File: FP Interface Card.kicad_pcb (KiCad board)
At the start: 6 copper layers, 90.2 x 101.1 mm, 40 parts, among them J100 ZX62-AB-5PA(31), P1 Card Edge for HSEC8-160-01-S-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, Q100 BC847BM3T5G, Q101 BC847BM3T5G, Q102 BC847BM3T5G, Q103 BC847BM3T5G, SW100 SW_Push_SPST, U100 AP2161W

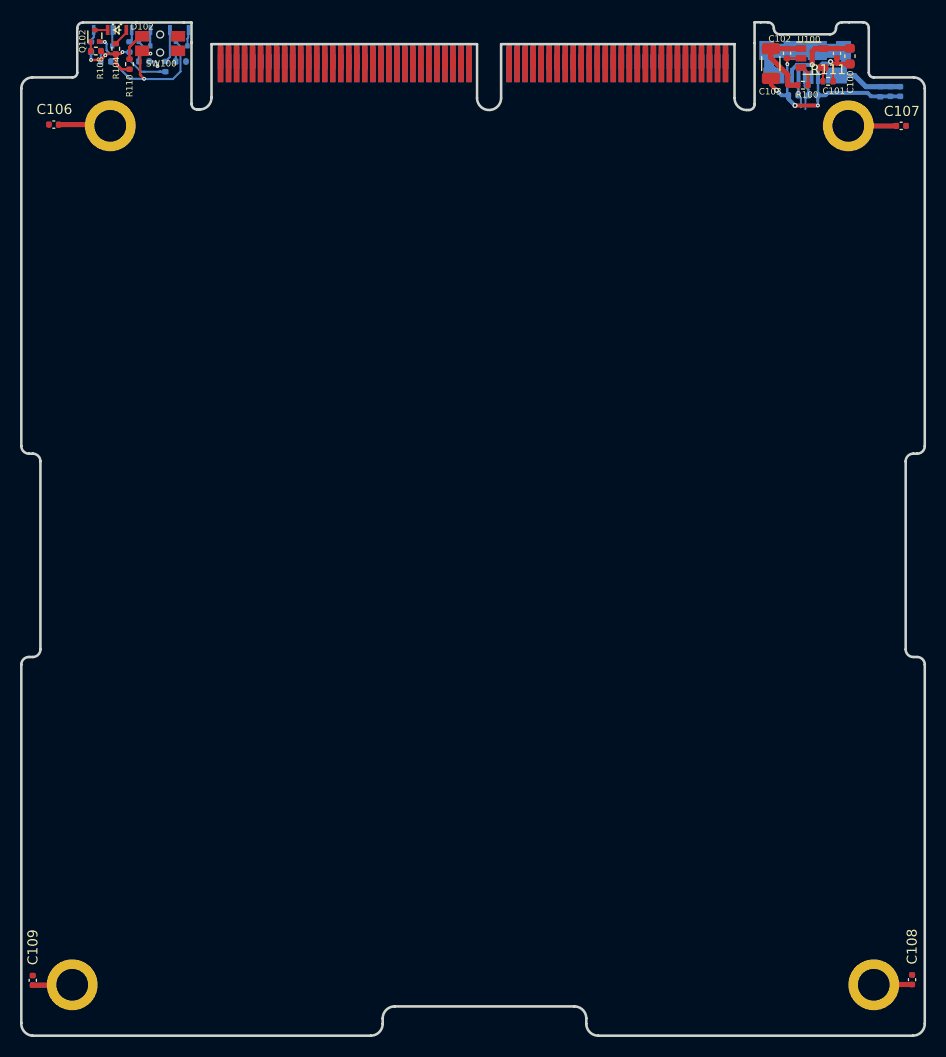
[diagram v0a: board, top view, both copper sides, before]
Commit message: 1
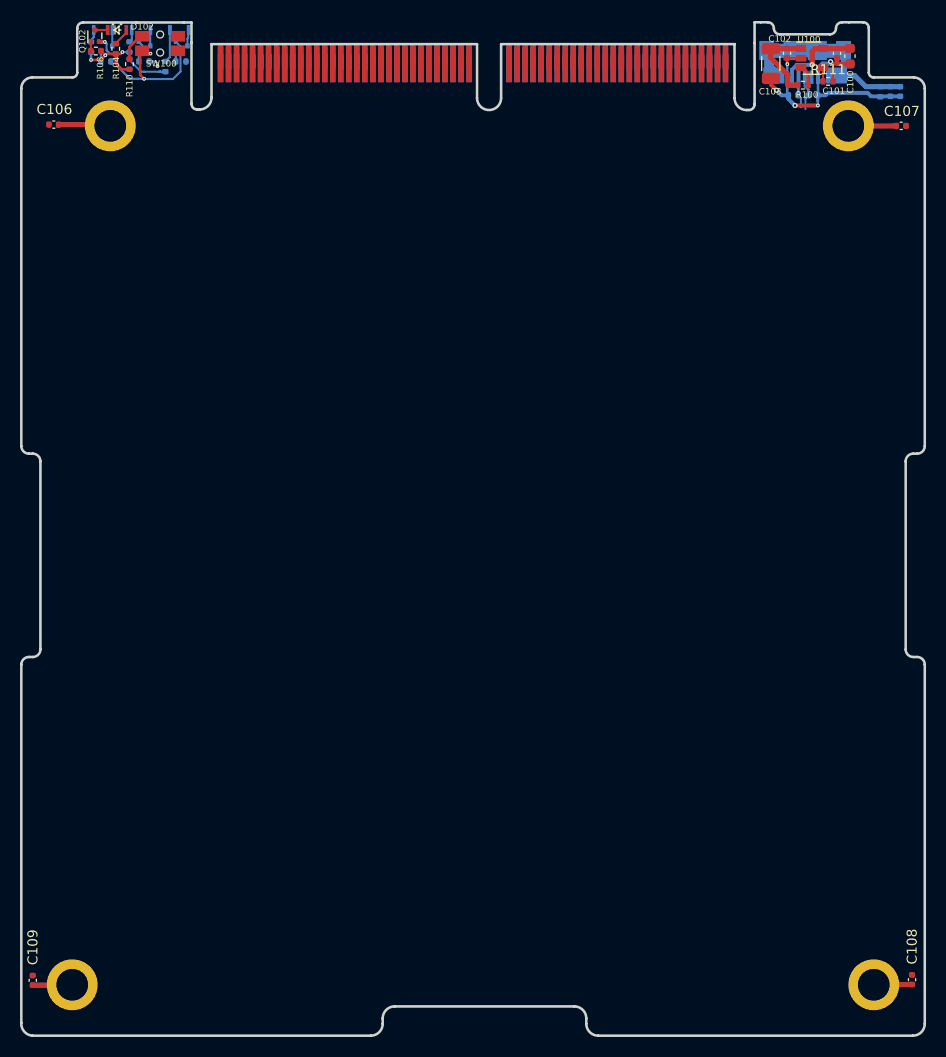
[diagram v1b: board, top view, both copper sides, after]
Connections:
- net /~BUS_RESET renamed /~{BUS_RESET}
- net /~USB_EN renamed /~{USB_EN}
- net /~USB_FLAG renamed /~{USB_FLAG}
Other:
- net class Default removed

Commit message: 1
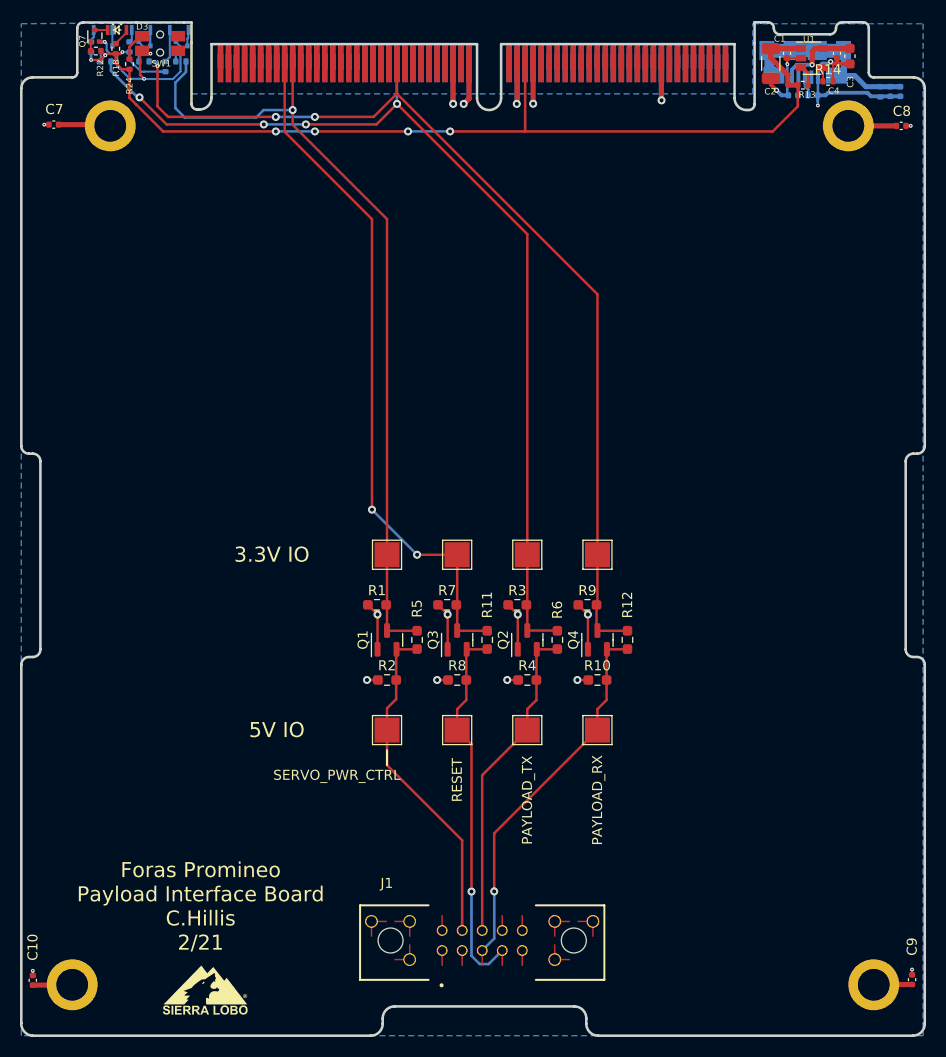
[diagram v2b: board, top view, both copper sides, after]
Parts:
- added G***: LOGO, payload-interface-board:Sierra_Lobo_Logo, F.Cu at (18.4, -4.55)
- added J1: T2M-105-01-X-D-TH-DS, payload-interface-board:SAMTEC_T2M-105-01-X-D-TH-DS, F.Cu at (46.0, -9.50)
- added Q1: Q_NMOS_GSD, Package_TO_SOT_SMD:SOT-23, F.Cu at (36.5, -39.5)
- added Q2: Q_NMOS_GSD, Package_TO_SOT_SMD:SOT-23, F.Cu at (50.5, -39.5)
- added Q3: Q_NMOS_GSD, Package_TO_SOT_SMD:SOT-23, F.Cu at (43.5, -39.5)
- added Q4: Q_NMOS_GSD, Package_TO_SOT_SMD:SOT-23, F.Cu at (57.5, -39.5)
- added R1: 10k, Resistor_SMD:R_0603_1608Metric_Pad0.98x0.95mm_HandSolder, F.Cu at (35.5, -43.0)
- added R10: 10k, Resistor_SMD:R_0603_1608Metric_Pad0.98x0.95mm_HandSolder, F.Cu at (57.5, -35.5)
- added R11: 0, Resistor_SMD:R_0603_1608Metric_Pad0.98x0.95mm_HandSolder, F.Cu at (46.5, -39.5)
- added R12: 0, Resistor_SMD:R_0603_1608Metric_Pad0.98x0.95mm_HandSolder, F.Cu at (60.5, -39.5)
- added R2: 10k, Resistor_SMD:R_0603_1608Metric_Pad0.98x0.95mm_HandSolder, F.Cu at (36.5, -35.5)
- added R3: 10k, Resistor_SMD:R_0603_1608Metric_Pad0.98x0.95mm_HandSolder, F.Cu at (49.5, -43.0)
- added R4: 10k, Resistor_SMD:R_0603_1608Metric_Pad0.98x0.95mm_HandSolder, F.Cu at (50.5, -35.5)
- added R5: 0, Resistor_SMD:R_0603_1608Metric_Pad0.98x0.95mm_HandSolder, F.Cu at (39.5, -39.5)
- added R6: 0, Resistor_SMD:R_0603_1608Metric_Pad0.98x0.95mm_HandSolder, F.Cu at (53.5, -39.5)
- added R7: 10k, Resistor_SMD:R_0603_1608Metric_Pad0.98x0.95mm_HandSolder, F.Cu at (42.5, -43.0)
- added R8: 10k, Resistor_SMD:R_0603_1608Metric_Pad0.98x0.95mm_HandSolder, F.Cu at (43.5, -35.5)
- added R9: 10k, Resistor_SMD:R_0603_1608Metric_Pad0.98x0.95mm_HandSolder, F.Cu at (56.5, -43.0)
- added TP1: TestPoint, TestPoint:TestPoint_Pad_2.5x2.5mm, F.Cu at (43.5, -48.0)
- added TP2: TestPoint, TestPoint:TestPoint_Pad_2.5x2.5mm, F.Cu at (36.5, -48.0)
- added TP3: TestPoint, TestPoint:TestPoint_Pad_2.5x2.5mm, F.Cu at (43.5, -30.5)
- added TP4: TestPoint, TestPoint:TestPoint_Pad_2.5x2.5mm, F.Cu at (36.5, -30.5)
- added TP5: TestPoint, TestPoint:TestPoint_Pad_2.5x2.5mm, F.Cu at (50.5, -48.0)
- added TP6: TestPoint, TestPoint:TestPoint_Pad_2.5x2.5mm, F.Cu at (57.5, -48.0)
- added TP7: TestPoint, TestPoint:TestPoint_Pad_2.5x2.5mm, F.Cu at (50.5, -30.5)
- added TP8: TestPoint, TestPoint:TestPoint_Pad_2.5x2.5mm, F.Cu at (57.5, -30.5)
- renumbered C102 to C1, C109 to C10, C103 to C2, C100 to C3, C101 to C4, C104 to C5, C105 to C6, C106 to C7, C107 to C8, C108 to C9, D100 to D1, D101 to D2, D102 to D3, D103 to D4, H100 to H1, H101 to H2, H102 to H3, H103 to H4, J100 to J2, Q100 to Q5, Q101 to Q6, Q102 to Q7, Q103 to Q8, R100 to R13, R111 to R14, R101 to R15, R102 to R16, R103 to R17, R104 to R18, R105 to R19, R106 to R20, R107 to R21, R108 to R22, R109 to R23, R110 to R24, SW100 to SW1, U100 to U1, Z100 to Z1, Z101 to Z2
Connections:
- net /SCK0 renamed /H1-21
- net /SDI0 renamed /H1-22
- net /SDO0 renamed /H1-23
- net /VCC_sys renamed +3V3
- C1 pad 2: /Blank-Card-Default/GND -> GND
- C10 pad 1: /Blank-Card-Default/GND -> GND
- C2 pad 2: /Blank-Card-Default/GND -> GND
- C3 pad 2: /Blank-Card-Default/GND -> GND
- C4 pad 2: /Blank-Card-Default/GND -> GND
- C5 pad 2: /Blank-Card-Default/GND -> GND
- C6 pad 2: /Blank-Card-Default/GND -> GND
- C7 pad 1: /Blank-Card-Default/GND -> GND
- C8 pad 1: /Blank-Card-Default/GND -> GND
- C9 pad 1: /Blank-Card-Default/GND -> GND
- J2 pad 4: Net-(J100-Pad4) -> unconnected-(J2-Pad4)
- J2 pad 5: /Blank-Card-Default/GND -> GND
- P1 pad 103: /GND -> GND
- P1 pad 104: /GND -> GND
- P1 pad 45: /URx0 -> /H1-19
- P1 pad 46: /UTx0 -> /H1-20
- P1 pad 59: /H2-25 -> +5V
- P1 pad 60: /H2-26 -> +5V
- P1 pad 67: /GND -> GND
- P1 pad 68: /GND -> GND
- P1 pad 72: /GND -> GND
- Q5 pad 2: /Blank-Card-Default/GND -> GND
- Q6 pad 2: /Blank-Card-Default/GND -> GND
- Q7 pad 2: /Blank-Card-Default/GND -> GND
- Q8 pad 2: /Blank-Card-Default/GND -> GND
- R14 pad 2: /Blank-Card-Default/GND -> GND
- R15 pad 2: /Blank-Card-Default/GND -> GND
- R20 pad 2: /USB_D+ -> /H1-19
- R21 pad 2: /USB_D- -> /H1-20
- R23 pad 2: /ORG_LED -> /H2-6
- SW1 pad 2: /GND -> GND
- U1 pad 2: /Blank-Card-Default/GND -> GND
- Z1 pad 2: /Blank-Card-Default/GND -> GND
- Z2 pad 2: /Blank-Card-Default/GND -> GND
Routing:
- net /H1-20: track 0.00 -> 98.0 mm, vias 0 -> 3
- net /H1-19: track 0.00 -> 97.2 mm, vias 0 -> 4
- net /H2-6: track 0.00 -> 80.6 mm, vias 0 -> 1
- net /5V_USB: track 22.5 -> 103.0 mm, vias 3 -> 7
- net GND: track 0.00 -> 70.9 mm, vias 0 -> 14
- net /H1-6: track 0.00 -> 68.7 mm, vias 0 -> 2
- net /RESET: track 0.00 -> 37.6 mm, vias 0 -> 1
- net /RXD: track 0.00 -> 37.3 mm, vias 0 -> 1
- net /Blank-Card-Default/GND: track 34.5 -> 0.00 mm, vias 5 -> 0
- net /SERVO_PWR_CTRL: track 0.00 -> 33.6 mm
- net /TXD: track 0.00 -> 32.4 mm
- net +3V3: track 0.00 -> 26.9 mm, vias 0 -> 5
- net /GND: track 20.9 -> 0.00 mm, vias 3 -> 0
- net +5V: track 0.00 -> 11.5 mm, vias 0 -> 5
- net /USB_D-: track 4.30 -> 1.82 mm, vias 1 -> 0
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- added copper zone on B.Cu, net +3V3
- added copper zone on In1.Cu, net +5V
- added copper zone on In2.Cu, net GND
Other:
- copper layers 6 -> 4
- board text added: "3.3V IO"
- board text added: "5V IO"
- board text added: "Foras Promineo Payload Interface Board C.Hillis 2/21"
- board text added: "PAYLOAD_RX"
- board text added: "PAYLOAD_TX"
- board text added: "RESET"
- board text added: "SERVO_PWR_CTRL"
